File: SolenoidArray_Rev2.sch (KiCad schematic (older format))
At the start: 112 parts, among them J1 Conn_01x02, J10 Conn_01x02, J11 Conn_01x02, J12 Conn_01x02, J13 Conn_01x02, J14 Conn_01x02, J15 Conn_01x02, J16 Power Daisy Chain_input, J17 Power Daisy Chain_Output, J18 Arduino Pins, J19 Screw_Terminal_01x02, J2 Conn_01x02, J3 Conn_01x02, J4 Conn_01x02, J5 Conn_01x02, J6 Conn_01x02, J7 Conn_01x02, J8 Conn_01x02, J9 Conn_01x02, Q1 AOD508, Q10 AOD508, Q11 AOD508, Q12 AOD508, Q13 AOD508, Q14 AOD508, Q15 AOD508, Q2 AOD508, Q3 AOD508, Q4 AOD508, Q5 AOD508, Q6 AOD508, Q7 AOD508, Q8 AOD508, Q9 AOD508

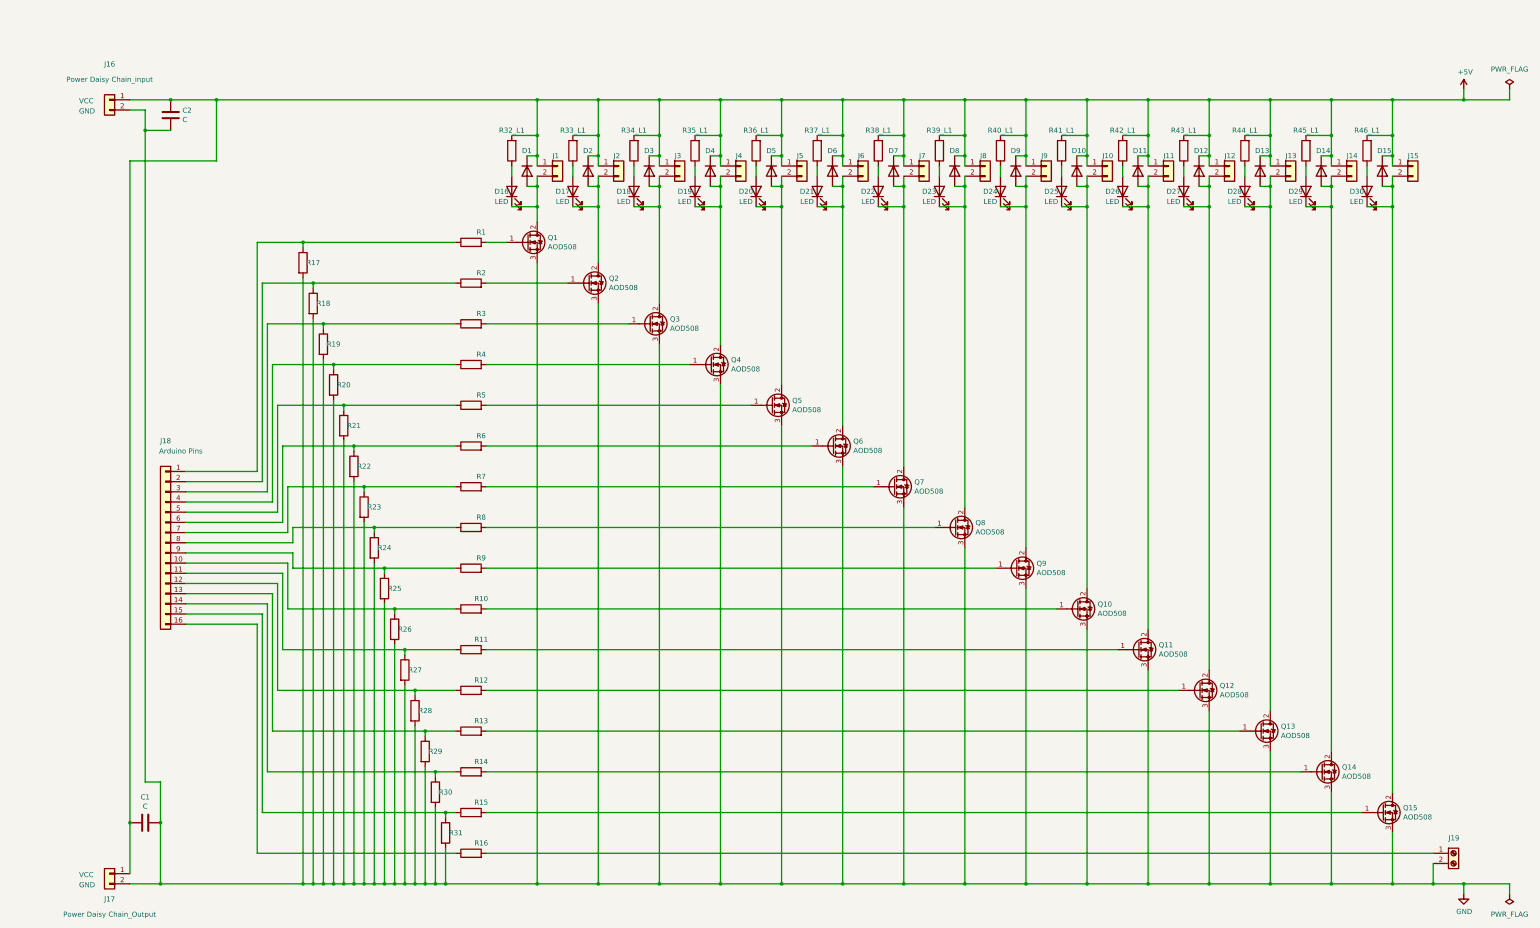
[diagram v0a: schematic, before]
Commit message: .
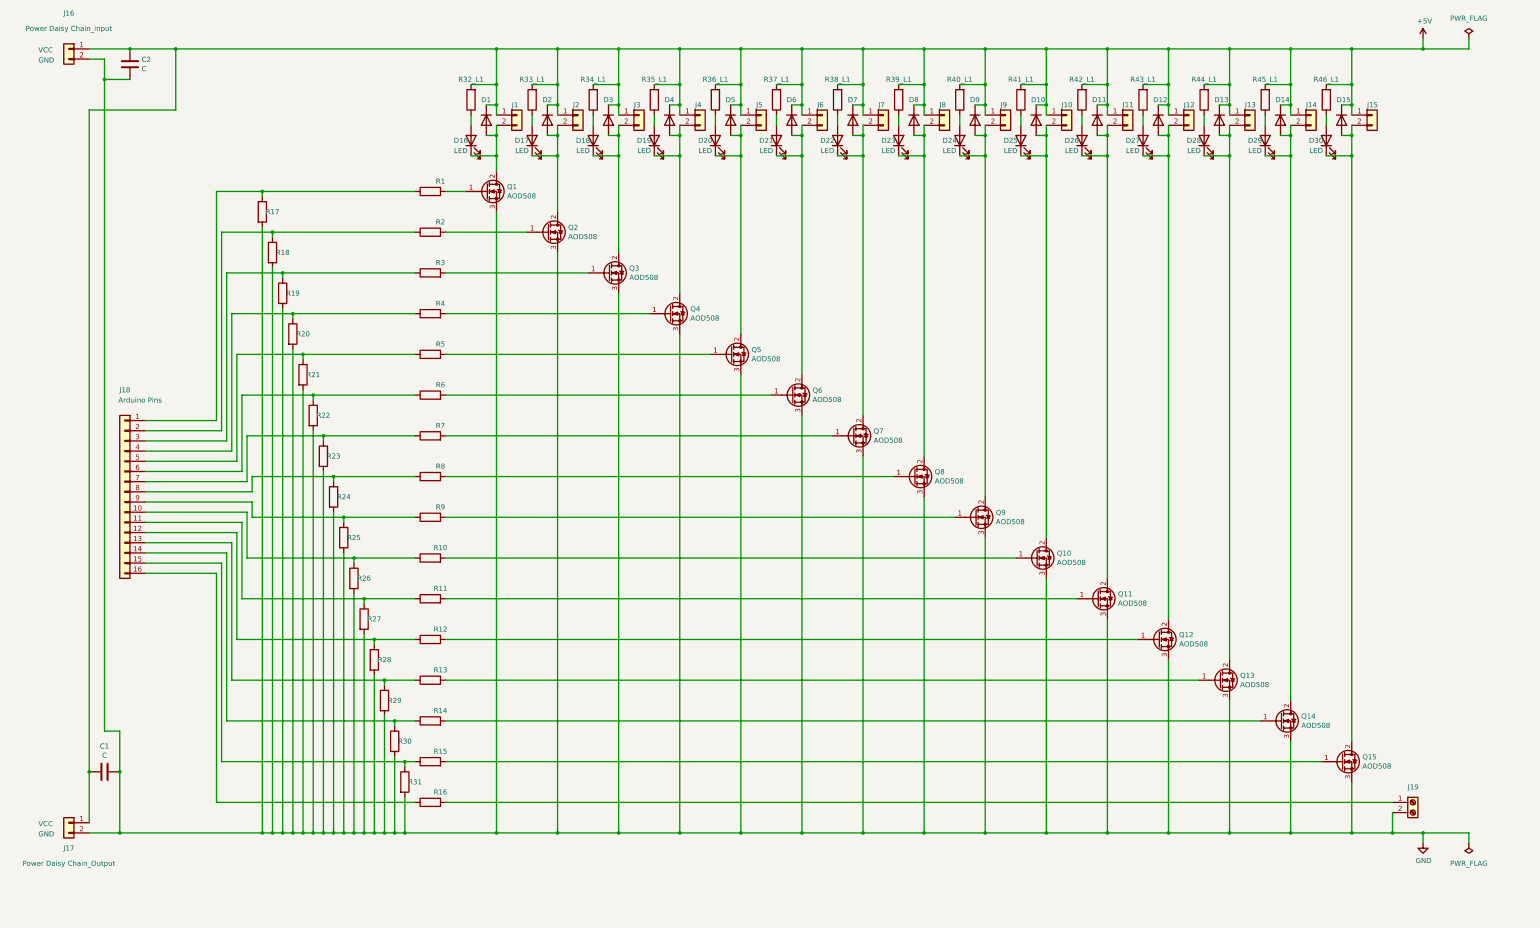
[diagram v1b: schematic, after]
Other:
- moved on the sheet: C1, C2, D1, D10, D11, D12, D13, D14, D15, D16, D17, D18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
